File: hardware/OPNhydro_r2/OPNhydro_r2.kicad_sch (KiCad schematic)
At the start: 164 parts, among them J2 MKDS, J3 BNC, J4 BNC, J5 BNC, M1 ESP32-C6-DEVKIT, M2 ATLAS_EZO_pH, M3 ATLAS_EZO_EC, M4 ATLAS_EZO_RTD, P1 MSTB_0.2", P10 ANKO_A200SX, P11 ANKO_A200SX, P12 ANKO_A200SX, P13 PB_1.25mm, P2 PHR_4, P3 MC_0.2", P4 DC40F-2460, P5 PHR_4, P6 MC_0.15", P7 XH_2.5mm, P8 XH_2.5mm, P9 XH_2.5mm, SW1 FLOAT, SW2 FLOAT, T1 AON6407, T2 BT3904, T3 IRLR2905, T4 BT3904, T5 AO3400A, U1 TPS62933, U2 AZ1117-3.3, U3 ADM3260, U4 ADM3260, U5 TMC2209, U6 TMC2209, U7 TMC2209

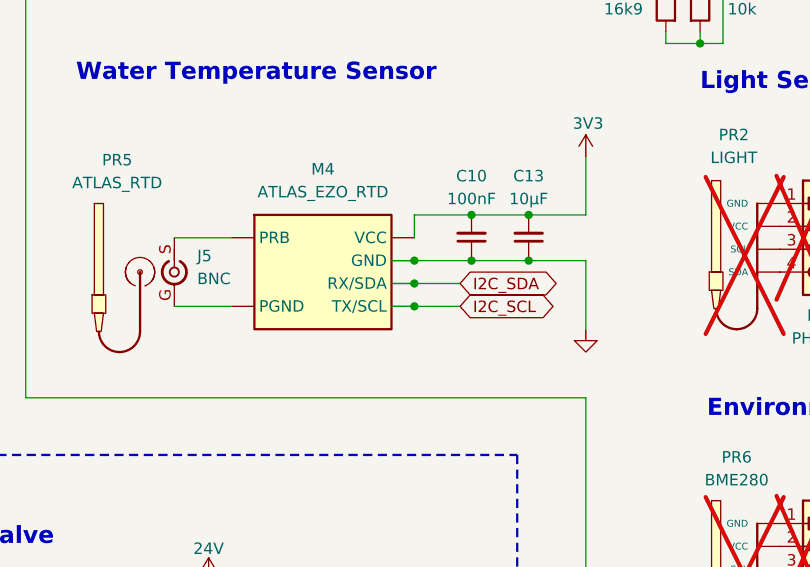
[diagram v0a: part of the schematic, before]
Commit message: update
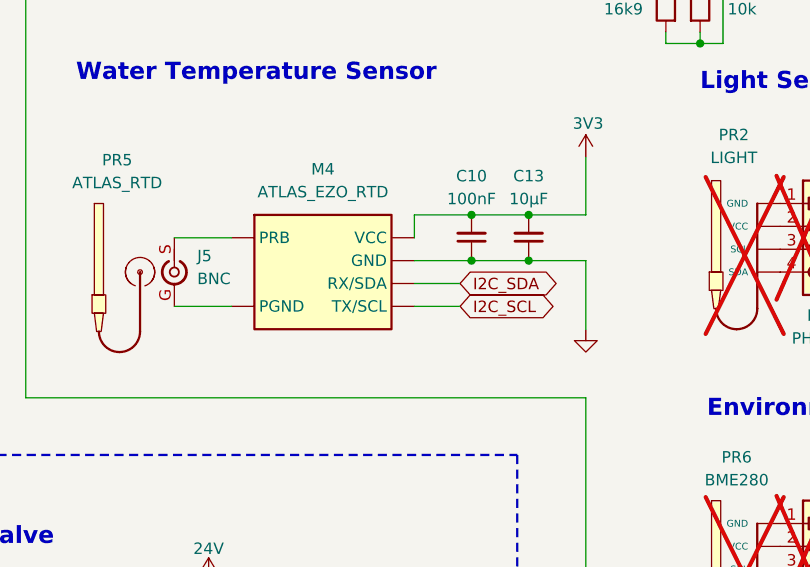
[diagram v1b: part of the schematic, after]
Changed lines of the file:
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@@
 	)
 	(junction
-		(at 161.29 195.58)
-		(diameter 0)
-		(color 0 0 0 0)
-	)
-	(junction
 		(at 290.83 212.09)
 		(diameter 0)
@@
 	)
 	(junction
+		(at 167.64 195.58)
+		(diameter 0)
+		(color 0 0 0 0)
+	)
+	(junction
 		(at 173.99 195.58)
 		(diameter 0)
@@
 	)
 	(junction
-		(at 161.29 198.12)
-		(diameter 0)
-		(color 0 0 0 0)
-	)
-	(junction
-		(at 161.29 200.66)
-		(diameter 0)
-		(color 0 0 0 0)
-	)
-	(junction
 		(at 189.23 95.25)
 		(diameter 0)
@@
 	)
 	(junction
-		(at 167.64 195.58)
-		(diameter 0)
-		(color 0 0 0 0)
-	)
-	(junction
 		(at 171.45 38.1)
 		(diameter 0)
@@
 	(wire
 		(pts
-			(xy 158.75 195.58) (xy 161.29 195.58)
-		)
-		(stroke
-			(width 0)
-			(type default)
-		)
-	)
-	(wire
-		(pts
 			(xy 233.68 105.41) (xy 238.76 105.41)
 		)
@@
 	(wire
 		(pts
+			(xy 161.29 198.12) (xy 166.37 198.12)
+		)
+		(stroke
+			(width 0)
+			(type default)
+		)
+	)
+	(wire
+		(pts
 			(xy 290.83 223.52) (xy 290.83 222.25)
 		)
@@
 	(wire
 		(pts
+			(xy 161.29 195.58) (xy 167.64 195.58)
+		)
+		(stroke
+			(width 0)
+			(type default)
+		)
+	)
+	(wire
+		(pts
 			(xy 36.83 104.14) (xy 44.45 104.14)
 		)
@@
 	(wire
 		(pts
-			(xy 161.29 195.58) (xy 167.64 195.58)
-		)
-		(stroke
-			(width 0)
-			(type default)
-		)
-	)
-	(wire
-		(pts
 			(xy 176.53 95.25) (xy 175.26 95.25)
 		)
@@
 	(wire
 		(pts
-			(xy 158.75 200.66) (xy 161.29 200.66)
-		)
-		(stroke
-			(width 0)
-			(type default)
-		)
-	)
-	(wire
-		(pts
 			(xy 189.23 162.56) (xy 189.23 156.21)
 		)
@@
 	(wire
 		(pts
-			(xy 161.29 200.66) (xy 166.37 200.66)
-		)
-		(stroke
-			(width 0)
-			(type default)
-		)
-	)
-	(wire
-		(pts
 			(xy 350.52 212.09) (xy 350.52 224.79)
 		)
@@
 	(wire
 		(pts
+			(xy 161.29 200.66) (xy 166.37 200.66)
+		)
+		(stroke
+			(width 0)
+			(type default)
+		)
+	)
+	(wire
+		(pts
 			(xy 167.64 190.5) (xy 173.99 190.5)
 		)
@@
 	(wire
 		(pts
-			(xy 161.29 198.12) (xy 166.37 198.12)
-		)
-		(stroke
-			(width 0)
-			(type default)
-		)
-	)
-	(wire
-		(pts
 			(xy 54.61 242.57) (xy 54.61 245.11)
 		)
@@
 	(wire
 		(pts
-			(xy 158.75 198.12) (xy 161.29 198.12)
-		)
-		(stroke
-			(width 0)
-			(type default)
-		)
-	)
-	(wire
-		(pts
 			(xy 163.83 148.59) (xy 163.83 156.21)
 		)
@@
 		)
 		(instances
-			(project ""
+			(project "OPNhydro_r2"
 				(path "/a0000000-0000-4000-8000-000000002687"
 					(reference "M4")
